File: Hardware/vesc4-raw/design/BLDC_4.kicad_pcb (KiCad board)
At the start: 4 copper layers, 38.5 x 65 mm, 127 parts, among them K1 SERVO, P1 HALL/Encoder, P101 CANBUS, P2 SWD, P3 PWR_COMM, P4 IN+, P5 IN-, P6 MOTOR1, P7 MOTOR2, P9 MOTOR3, Q1 IRFS7530, Q2 IRFS7530, Q3 IRFS7530, Q4 IRFS7530, Q5 IRFS7530, Q6 IRFS7530, U1 STM32F40X_LQFP64, U2 TC2117, U3 DRV8302, U401 SN65HVD232, X1 MINI-USB-SHIELD-32005-201, X2 8MHz 10ppm

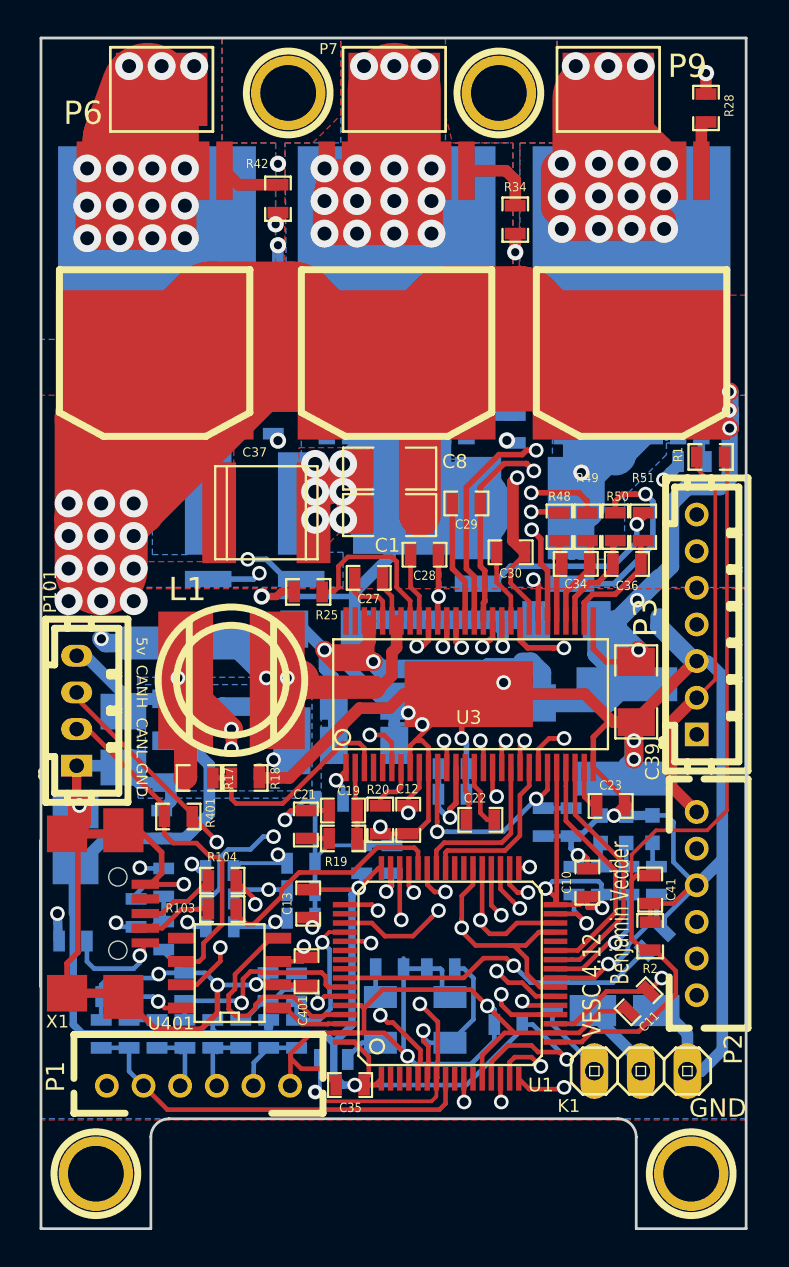
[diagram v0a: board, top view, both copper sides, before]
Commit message: sebelum-coba-fix
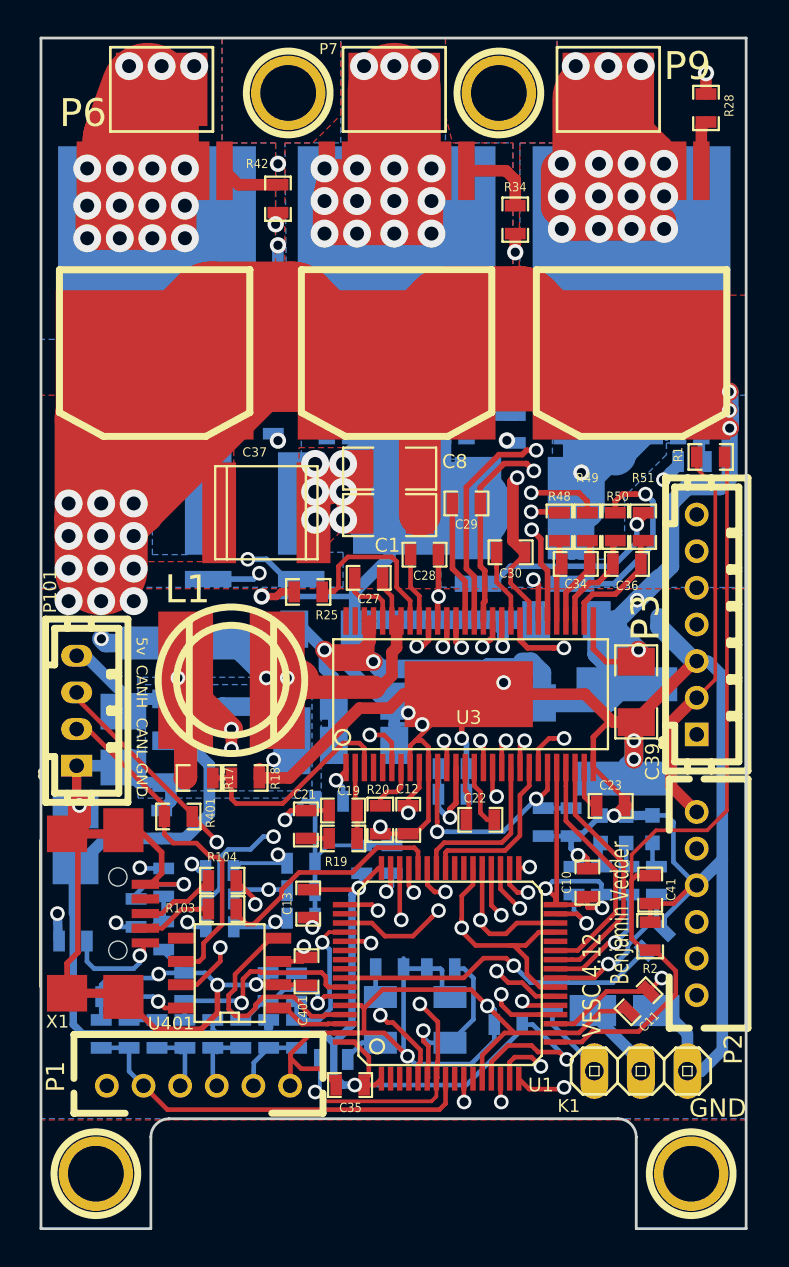
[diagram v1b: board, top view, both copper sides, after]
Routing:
- added copper zone on In1.Cu, net /Mosfet driver/H1_VS
- added copper zone on In2.Cu, net /Mosfet driver/H1_VS
- added copper zone on In1.Cu, net /Mosfet driver/H2_VS
- added copper zone on In2.Cu, net /Mosfet driver/H2_VS
- added copper zone on In1.Cu, net /Mosfet driver/H3_VS
- added copper zone on In2.Cu, net /Mosfet driver/H3_VS
- added copper zone on In1.Cu, net GND
- added copper zone on In2.Cu, net GND
- removed copper zone on GND, net /Mosfet driver/H1_VS
- removed copper zone on GND2, net /Mosfet driver/H1_VS
- removed copper zone on GND, net /Mosfet driver/H2_VS
- removed copper zone on GND2, net /Mosfet driver/H2_VS
- removed copper zone on GND, net /Mosfet driver/H3_VS
- removed copper zone on GND2, net /Mosfet driver/H3_VS
- removed copper zone on GND, net GND
- removed copper zone on GND2, net GND
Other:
- net class Default removed
